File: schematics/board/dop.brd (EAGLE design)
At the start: 65.8 x 65.8 mm, 78 parts

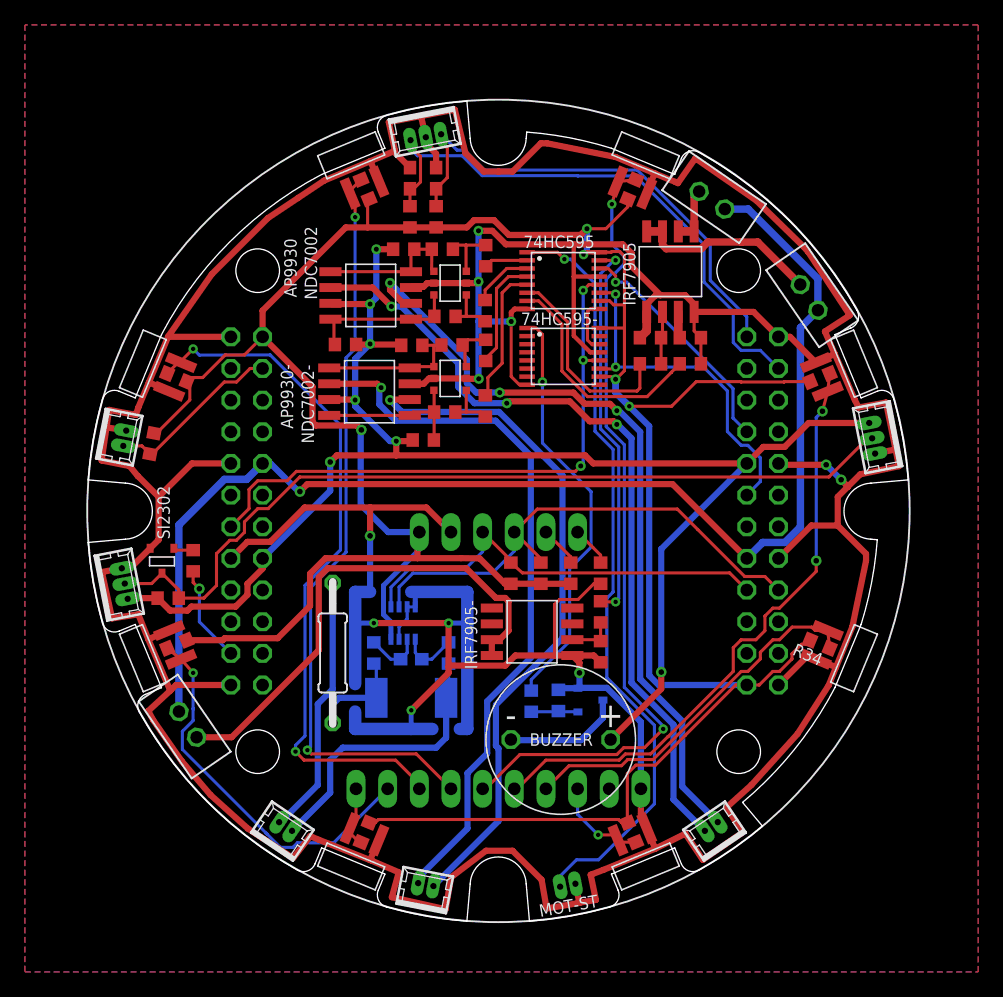
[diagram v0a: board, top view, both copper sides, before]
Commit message: Подготовлена плата dop
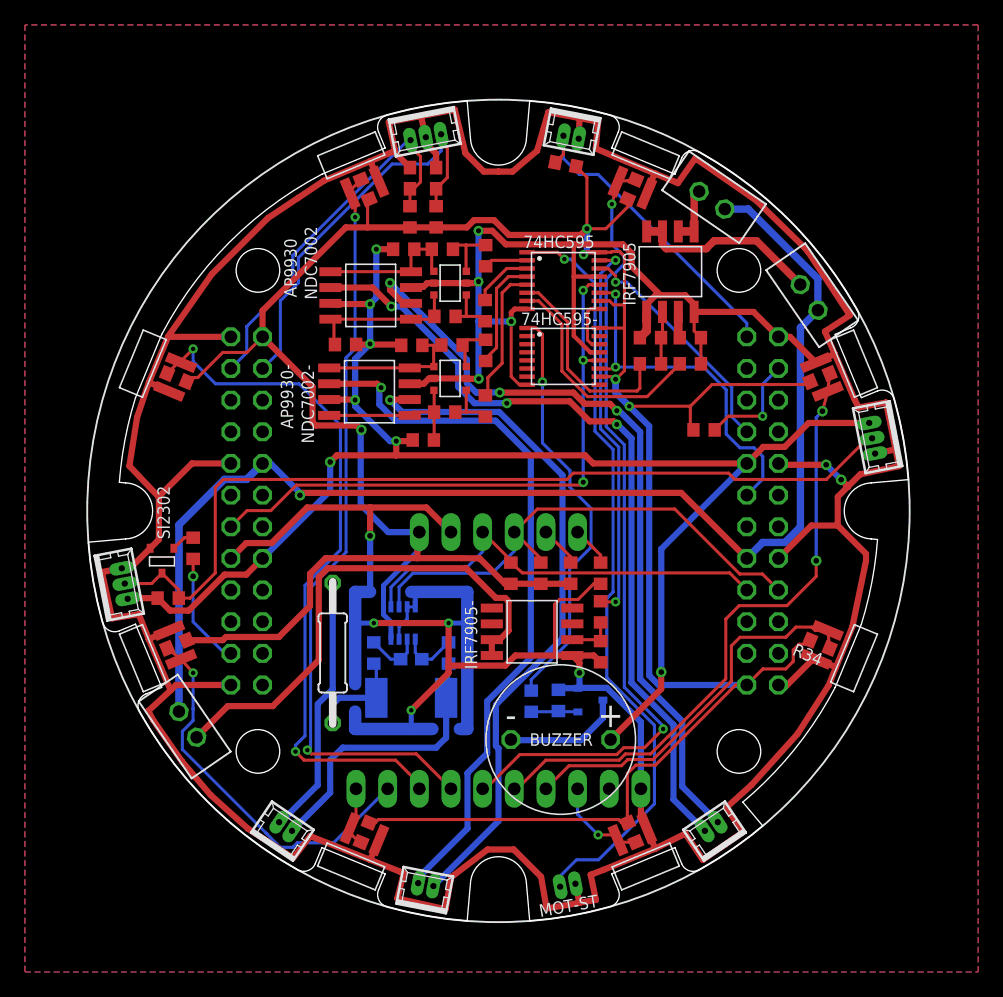
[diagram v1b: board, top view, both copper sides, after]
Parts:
- added R40: 10k, rcl:R0603
- moved PHOTO 43.8 mm to (38.9, 63.4), turned to 169 degrees
- moved R39 40.0 mm to (38.4, 60.8), turned to 349 degrees
- moved R41 1.00 mm to (8.50, 30.0)
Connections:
- removed net PA6: A.21
- removed net PC5: A.20
- new net SWITCH: B.22, R40.1
- net 3V3: now also R40.2
- net ENCOD_A: now also A.21; no longer B.22
- net ENCOD_B: now also A.22; no longer B.23
- net FOTO9: now also B.23; no longer A.22
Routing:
- net ENCOD_A: track 46.9 -> 30.6 mm
- net FOTO9: track 14.3 -> 25.5 mm
- net SWITCH: track 0.00 -> 8.66 mm, vias 0 -> 1
- net ENCOD_B: track 40.3 -> 32.8 mm
- net N$23: track 68.8 -> 71.3 mm
- net 3V3: track 238.6 -> 240.7 mm
- net FOTO2: track 29.9 -> 31.2 mm
- net LED: track 7.84 -> 9.13 mm
- net FOTO3: track 49.4 -> 50.7 mm
- net 5V: track 126.4 -> 125.4 mm
- net FOTO6: track 56.5 -> 57.1 mm
- net SCK: track 28.6 -> 29.1 mm
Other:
- outline, holes or cut-outs redrawn
